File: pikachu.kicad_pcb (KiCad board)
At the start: 2 copper layers, 35.3 x 35.3 mm, 1 part

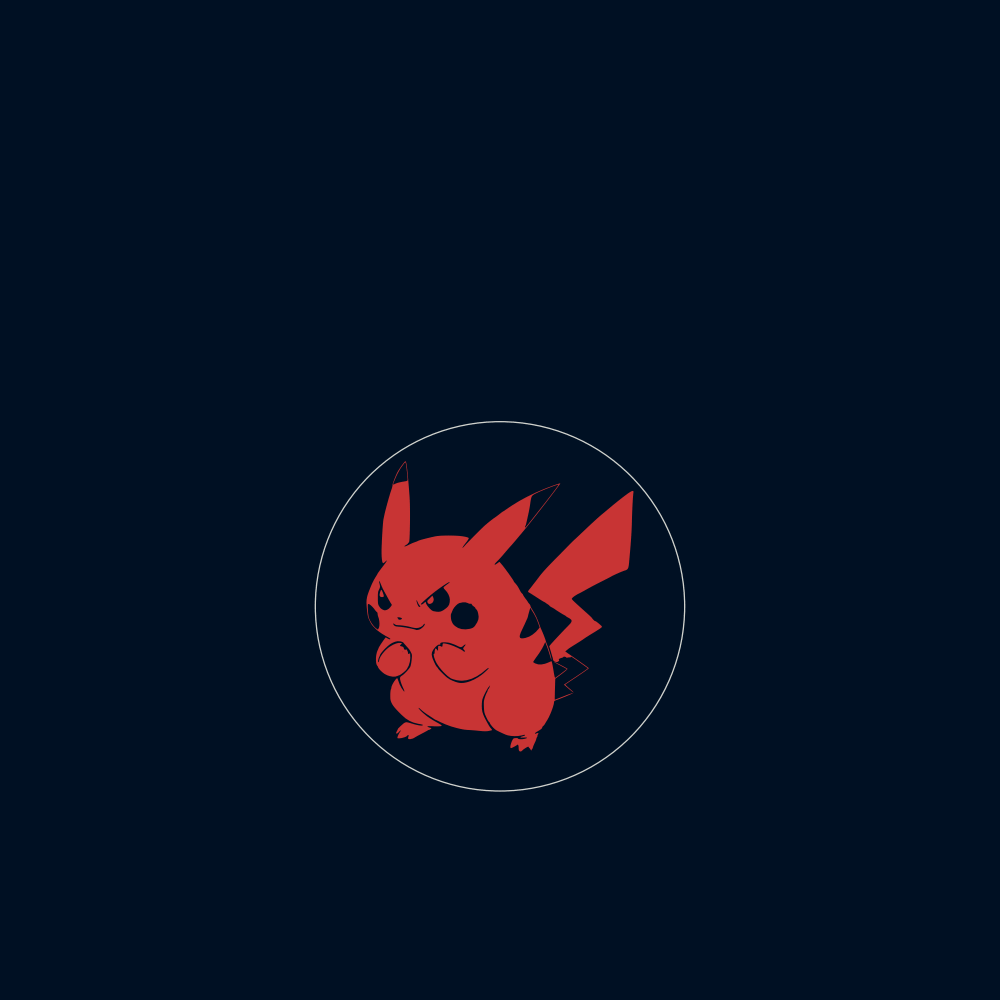
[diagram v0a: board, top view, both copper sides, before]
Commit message: added rays
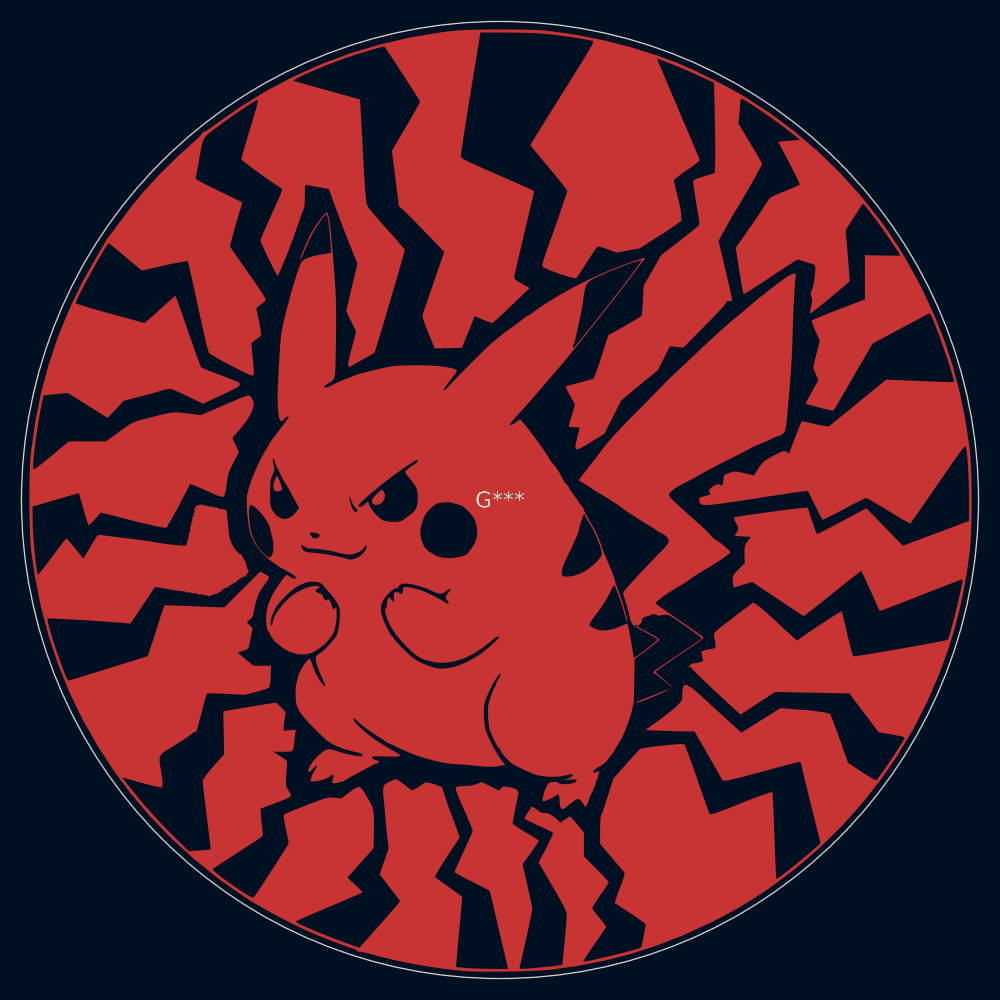
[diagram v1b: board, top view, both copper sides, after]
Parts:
- removed the G*** at (137.7, 96.6)
- added G***: LOGO, pikachus:pikachu_9090_rays, F.Cu at (139.7, 86.4)
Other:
- board size 35.3 x 35.3 mm -> 91.4 x 91.4 mm
